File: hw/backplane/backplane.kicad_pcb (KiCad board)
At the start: 2 copper layers, 219.2 x 20.9 mm, 27 parts, among them J1 out1, J10 conn5, J11 conn6, J12 out6, J13 Screw_Terminal_01x02, J2 out2, J3 conn2, J4 conn3, J5 conn1, J6 out3, J7 conn4, J8 out4, J9 out5

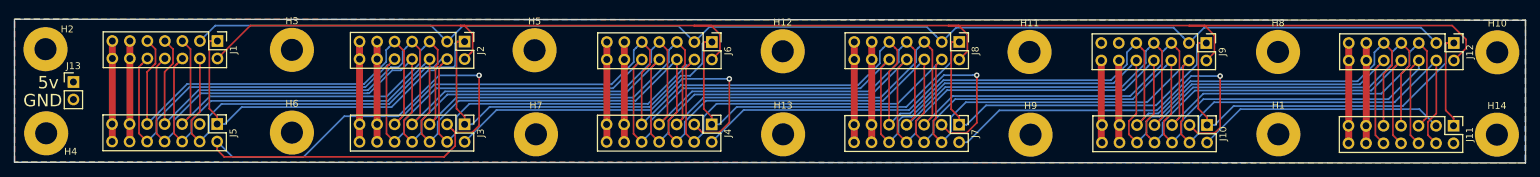
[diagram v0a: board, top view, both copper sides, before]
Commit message: updates
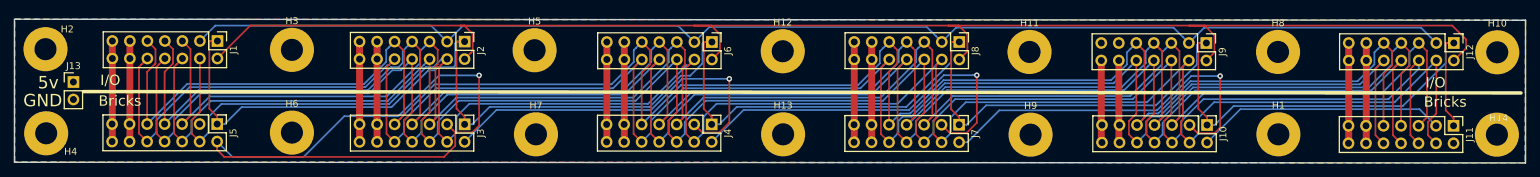
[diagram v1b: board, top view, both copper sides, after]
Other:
- board text added: "Bricks"
- board text added: "I/O"
